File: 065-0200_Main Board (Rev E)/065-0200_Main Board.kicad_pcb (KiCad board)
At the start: 2 copper layers, 152.5 x 54.6 mm, 22 parts, among them J1 UJ32-C-H-G-H2-SMT-TR, J2 0022035025, J3 0022035025, J4 custom_3p_2mm, J5 custom_2p_2mm, SW1 3-1437565-0, U1 QRE1113GR, U2 QRE1113GR, U3 QRE1113GR, U4 BM833, U5 2SMPP03

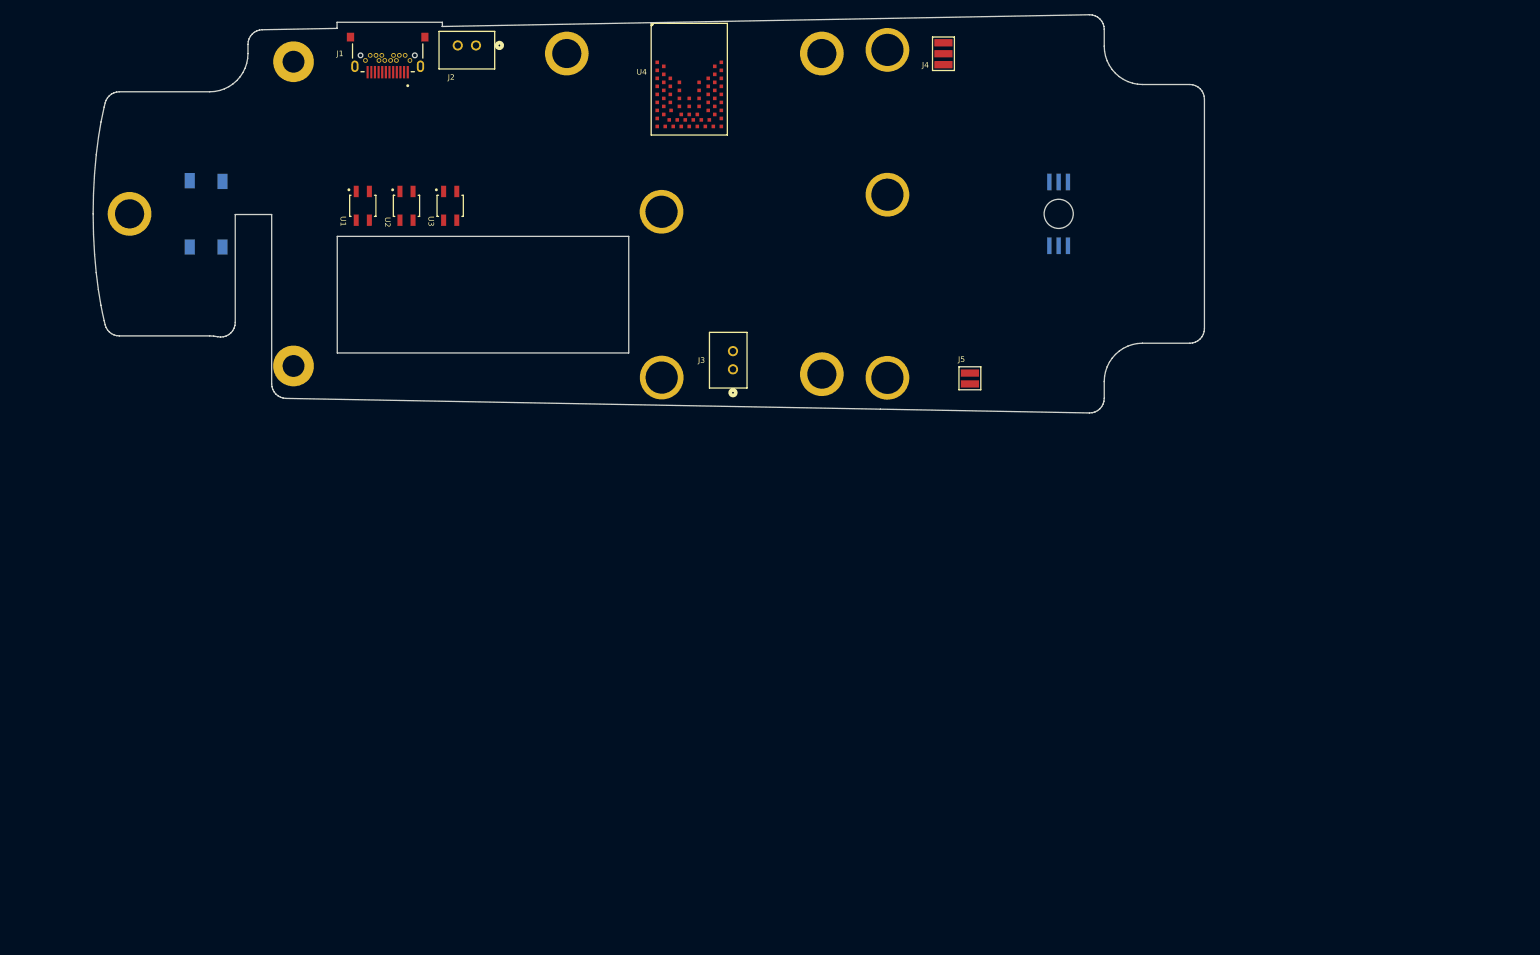
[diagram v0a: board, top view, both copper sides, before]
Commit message: Place all 155 remaining components on B.Cu off-board
Components grouped by circuit function below/around the board outline,
ready for manual placement. All on B.Cu with layers flipped F↔B.

Co-Authored-By: Claude Sonnet 4.6 <noreply@anthropic.com>
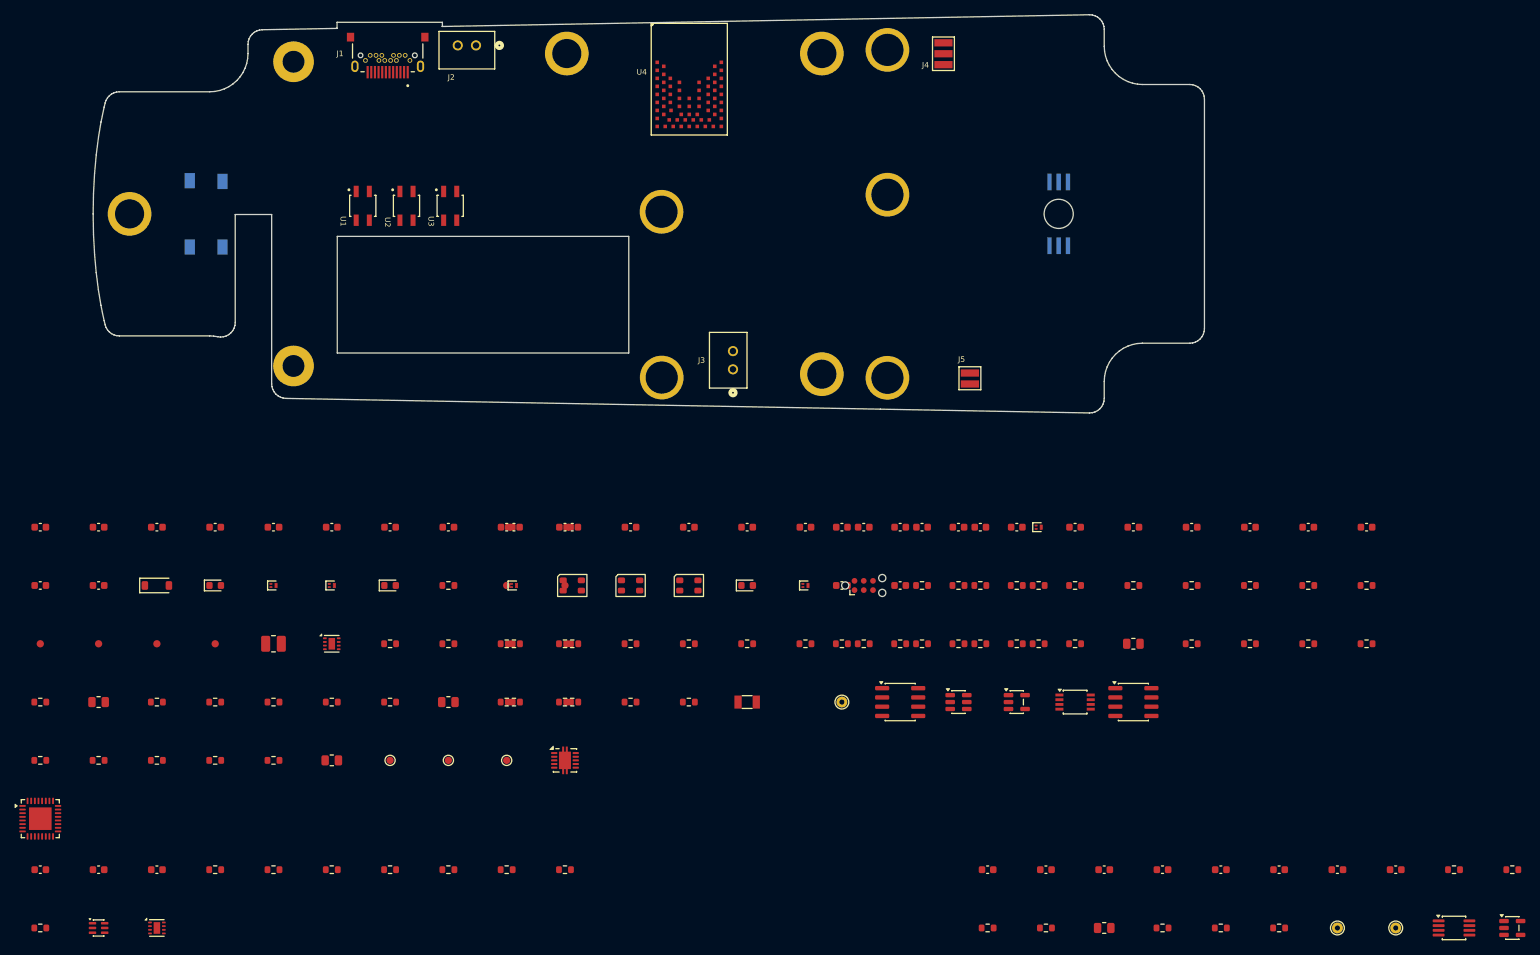
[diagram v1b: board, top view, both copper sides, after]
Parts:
- added C1: C_0603_1608Metric, Capacitor_SMD:C_0603_1608Metric, B.Cu at (65.0, 148.0)
- added C10: C_0603_1608Metric, Capacitor_SMD:C_0603_1608Metric, B.Cu at (73.0, 148.0)
- added C11: C_0603_1608Metric, Capacitor_SMD:C_0603_1608Metric, B.Cu at (195.0, 195.0)
- added C12: C_0603_1608Metric, Capacitor_SMD:C_0603_1608Metric, B.Cu at (203.0, 195.0)
- added C13: C_0603_1608Metric, Capacitor_SMD:C_0603_1608Metric, B.Cu at (211.0, 195.0)
- added C14: C_0603_1608Metric, Capacitor_SMD:C_0603_1608Metric, B.Cu at (175.0, 148.0)
- added C15: C_0603_1608Metric, Capacitor_SMD:C_0603_1608Metric, B.Cu at (183.0, 148.0)
- added C16: C_0603_1608Metric, Capacitor_SMD:C_0603_1608Metric, B.Cu at (219.0, 195.0)
- added C17: C_0603_1608Metric, Capacitor_SMD:C_0603_1608Metric, B.Cu at (191.0, 148.0)
- added C18: C_0603_1608Metric, Capacitor_SMD:C_0603_1608Metric, B.Cu at (199.0, 148.0)
- added C19: C_0603_1608Metric, Capacitor_SMD:C_0603_1608Metric, B.Cu at (207.0, 148.0)
- added C2: C_0603_1608Metric, Capacitor_SMD:C_0603_1608Metric, B.Cu at (81.0, 148.0)
- added C20: C_0603_1608Metric, Capacitor_SMD:C_0603_1608Metric, B.Cu at (215.0, 148.0)
- added C21: C_0603_1608Metric, Capacitor_SMD:C_0603_1608Metric, B.Cu at (227.0, 195.0)
- added C22: C_0603_1608Metric, Capacitor_SMD:C_0603_1608Metric, B.Cu at (223.0, 148.0)
- added C23: C_0603_1608Metric, Capacitor_SMD:C_0603_1608Metric, B.Cu at (231.0, 148.0)
- added C24: C_0603_1608Metric, Capacitor_SMD:C_0603_1608Metric, B.Cu at (235.0, 195.0)
- added C25: C_0603_1608Metric, Capacitor_SMD:C_0603_1608Metric, B.Cu at (243.0, 195.0)
- added C26: C_0603_1608Metric, Capacitor_SMD:C_0603_1608Metric, B.Cu at (239.0, 148.0)
- added C27: C_0603_1608Metric, Capacitor_SMD:C_0603_1608Metric, B.Cu at (247.0, 148.0)
- added C28: C_0603_1608Metric, Capacitor_SMD:C_0603_1608Metric, B.Cu at (251.0, 195.0)
- added C29: C_0603_1608Metric, Capacitor_SMD:C_0603_1608Metric, B.Cu at (175.0, 156.0)
- added C3: C_0603_1608Metric, Capacitor_SMD:C_0603_1608Metric, B.Cu at (130.0, 148.0)
- added C30: C_0603_1608Metric, Capacitor_SMD:C_0603_1608Metric, B.Cu at (89.0, 148.0)
- added C31: C_0603_1608Metric, Capacitor_SMD:C_0603_1608Metric, B.Cu at (97.0, 148.0)
- added C32: C_0603_1608Metric, Capacitor_SMD:C_0603_1608Metric, B.Cu at (183.0, 156.0)
- added C33: C_0603_1608Metric, Capacitor_SMD:C_0603_1608Metric, B.Cu at (105.0, 148.0)
- added C34: C_0603_1608Metric, Capacitor_SMD:C_0603_1608Metric, B.Cu at (113.0, 148.0)
- added C35: C_0603_1608Metric, Capacitor_SMD:C_0603_1608Metric, B.Cu at (121.0, 148.0)
- added C36: C_0603_1608Metric, Capacitor_SMD:C_0603_1608Metric, B.Cu at (129.0, 148.0)
- added C37: C_0603_1608Metric, Capacitor_SMD:C_0603_1608Metric, B.Cu at (137.0, 148.0)
- added C38: C_0603_1608Metric, Capacitor_SMD:C_0603_1608Metric, B.Cu at (138.0, 148.0)
- added C39: C_0603_1608Metric, Capacitor_SMD:C_0603_1608Metric, B.Cu at (146.0, 148.0)
- added C4: C_0603_1608Metric, Capacitor_SMD:C_0603_1608Metric, B.Cu at (154.0, 148.0)
- added C40: C_0603_1608Metric, Capacitor_SMD:C_0603_1608Metric, B.Cu at (162.0, 148.0)
- added C41: C_0603_1608Metric, Capacitor_SMD:C_0603_1608Metric, B.Cu at (65.0, 195.0)
- added C42: C_0603_1608Metric, Capacitor_SMD:C_0603_1608Metric, B.Cu at (73.0, 195.0)
- added C43: C_0603_1608Metric, Capacitor_SMD:C_0603_1608Metric, B.Cu at (81.0, 195.0)
- added C44: C_0603_1608Metric, Capacitor_SMD:C_0603_1608Metric, B.Cu at (65.0, 156.0)
- added C5: C_0603_1608Metric, Capacitor_SMD:C_0603_1608Metric, B.Cu at (170.0, 148.0)
- added C6: C_0603_1608Metric, Capacitor_SMD:C_0603_1608Metric, B.Cu at (178.0, 148.0)
- added C7: C_0603_1608Metric, Capacitor_SMD:C_0603_1608Metric, B.Cu at (186.0, 148.0)
- added C8: C_0603_1608Metric, Capacitor_SMD:C_0603_1608Metric, B.Cu at (194.0, 148.0)
- added C9: C_0603_1608Metric, Capacitor_SMD:C_0603_1608Metric, B.Cu at (73.0, 156.0)
- added D1: D_SOD-123, Diode_SMD:D_SOD-123, B.Cu at (81.0, 156.0)
- added D10: SOT-883, Package_TO_SOT_SMD:SOT-883, B.Cu at (202.0, 148.0)
- added D11: SOT-883, Package_TO_SOT_SMD:SOT-883, B.Cu at (130.0, 156.0)
- added D12: LED_0603_1608Metric, LED_SMD:LED_0603_1608Metric, B.Cu at (89.0, 156.0)
- added D2: SOT-883, Package_TO_SOT_SMD:SOT-883, B.Cu at (97.0, 156.0)
- added D3: SOT-883, Package_TO_SOT_SMD:SOT-883, B.Cu at (105.0, 156.0)
- added D4: LED_Cree-PLCC4_3.2x2.8mm_CCW, LED_SMD:LED_Cree-PLCC4_3.2x2.8mm_CCW, B.Cu at (138.0, 156.0)
- added D5: LED_Cree-PLCC4_3.2x2.8mm_CCW, LED_SMD:LED_Cree-PLCC4_3.2x2.8mm_CCW, B.Cu at (146.0, 156.0)
- added D6: LED_Cree-PLCC4_3.2x2.8mm_CCW, LED_SMD:LED_Cree-PLCC4_3.2x2.8mm_CCW, B.Cu at (154.0, 156.0)
- added D7: LED_0603_1608Metric, LED_SMD:LED_0603_1608Metric, B.Cu at (113.0, 156.0)
- added D8: LED_0603_1608Metric, LED_SMD:LED_0603_1608Metric, B.Cu at (162.0, 156.0)
- added D9: SOT-883, Package_TO_SOT_SMD:SOT-883, B.Cu at (170.0, 156.0)
- added F1: R_0603_1608Metric, Resistor_SMD:R_0603_1608Metric, B.Cu at (121.0, 156.0)
- added FD1: Fiducial_1mm_Mask2mm, Fiducial:Fiducial_1mm_Mask2mm, B.Cu at (129.0, 156.0)
- added FD2: Fiducial_1mm_Mask2mm, Fiducial:Fiducial_1mm_Mask2mm, B.Cu at (137.0, 156.0)
- added FD3: Fiducial_1mm_Mask2mm, Fiducial:Fiducial_1mm_Mask2mm, B.Cu at (65.0, 164.0)
- added FD4: Fiducial_1mm_Mask2mm, Fiducial:Fiducial_1mm_Mask2mm, B.Cu at (73.0, 164.0)
- added FD5: Fiducial_1mm_Mask2mm, Fiducial:Fiducial_1mm_Mask2mm, B.Cu at (81.0, 164.0)
- added FD6: Fiducial_1mm_Mask2mm, Fiducial:Fiducial_1mm_Mask2mm, B.Cu at (89.0, 164.0)
- added J6: Tag-Connect_TC2030-IDC-NL_2x03_P1.27mm_Vertical, Connector:Tag-Connect_TC2030-IDC-NL_2x03_P1.27mm_Vertical, B.Cu at (178.0, 156.0)
- added L1: L_1008_2520Metric, Inductor_SMD:L_1008_2520Metric, B.Cu at (97.0, 164.0)
- added Q1: WSON-8-1EP_2x2mm_P0.5mm_EP0.9x1.6mm, Package_SON:WSON-8-1EP_2x2mm_P0.5mm_EP0.9x1.6mm, B.Cu at (105.0, 164.0)
- added R1: R_0603_1608Metric, Resistor_SMD:R_0603_1608Metric, B.Cu at (113.0, 164.0)
- added R10: R_0603_1608Metric, Resistor_SMD:R_0603_1608Metric, B.Cu at (186.0, 156.0)
- added R11: R_0603_1608Metric, Resistor_SMD:R_0603_1608Metric, B.Cu at (194.0, 156.0)
- added R12: R_0603_1608Metric, Resistor_SMD:R_0603_1608Metric, B.Cu at (202.0, 156.0)
- added R13: R_0603_1608Metric, Resistor_SMD:R_0603_1608Metric, B.Cu at (130.0, 164.0)
- added R14: R_0603_1608Metric, Resistor_SMD:R_0603_1608Metric, B.Cu at (138.0, 164.0)
- added R15: R_0603_1608Metric, Resistor_SMD:R_0603_1608Metric, B.Cu at (146.0, 164.0)
- added R16: R_0603_1608Metric, Resistor_SMD:R_0603_1608Metric, B.Cu at (154.0, 164.0)
- added R17: R_0603_1608Metric, Resistor_SMD:R_0603_1608Metric, B.Cu at (162.0, 164.0)
- added R18: R_0603_1608Metric, Resistor_SMD:R_0603_1608Metric, B.Cu at (191.0, 156.0)
- added R19: R_0603_1608Metric, Resistor_SMD:R_0603_1608Metric, B.Cu at (199.0, 156.0)
- added R2: R_0603_1608Metric, Resistor_SMD:R_0603_1608Metric, B.Cu at (121.0, 164.0)
- added R20: R_0603_1608Metric, Resistor_SMD:R_0603_1608Metric, B.Cu at (259.0, 195.0)
- added R21: R_0603_1608Metric, Resistor_SMD:R_0603_1608Metric, B.Cu at (267.0, 195.0)
- added R22: R_0603_1608Metric, Resistor_SMD:R_0603_1608Metric, B.Cu at (207.0, 156.0)
- added R23: R_0603_1608Metric, Resistor_SMD:R_0603_1608Metric, B.Cu at (195.0, 203.0)
- added R24: R_0603_1608Metric, Resistor_SMD:R_0603_1608Metric, B.Cu at (203.0, 203.0)
- added R25: R_0603_1608Metric, Resistor_SMD:R_0603_1608Metric, B.Cu at (215.0, 156.0)
- added R26: R_0603_1608Metric, Resistor_SMD:R_0603_1608Metric, B.Cu at (223.0, 156.0)
- added R27: R_0603_1608Metric, Resistor_SMD:R_0603_1608Metric, B.Cu at (231.0, 156.0)
- added R28: R_0603_1608Metric, Resistor_SMD:R_0603_1608Metric, B.Cu at (239.0, 156.0)
- added R29: R_0603_1608Metric, Resistor_SMD:R_0603_1608Metric, B.Cu at (247.0, 156.0)
- added R3: R_0603_1608Metric, Resistor_SMD:R_0603_1608Metric, B.Cu at (129.0, 164.0)
- added R30: R_0603_1608Metric, Resistor_SMD:R_0603_1608Metric, B.Cu at (175.0, 164.0)
- added R31: R_0603_1608Metric, Resistor_SMD:R_0603_1608Metric, B.Cu at (183.0, 164.0)
- added R32: R_0603_1608Metric, Resistor_SMD:R_0603_1608Metric, B.Cu at (191.0, 164.0)
- added R33: R_0603_1608Metric, Resistor_SMD:R_0603_1608Metric, B.Cu at (199.0, 164.0)
- added R34: R_0805_2012Metric, Resistor_SMD:R_0805_2012Metric, B.Cu at (211.0, 203.0)
- added R35: R_0603_1608Metric, Resistor_SMD:R_0603_1608Metric, B.Cu at (207.0, 164.0)
- added R36: R_0805_2012Metric, Resistor_SMD:R_0805_2012Metric, B.Cu at (215.0, 164.0)
- added R37: R_0603_1608Metric, Resistor_SMD:R_0603_1608Metric, B.Cu at (219.0, 203.0)
- added R38: R_0603_1608Metric, Resistor_SMD:R_0603_1608Metric, B.Cu at (223.0, 164.0)
- added R39: R_0603_1608Metric, Resistor_SMD:R_0603_1608Metric, B.Cu at (231.0, 164.0)
- added R4: R_0603_1608Metric, Resistor_SMD:R_0603_1608Metric, B.Cu at (170.0, 164.0)
- added R40: R_0603_1608Metric, Resistor_SMD:R_0603_1608Metric, B.Cu at (137.0, 164.0)
- added R41: R_0603_1608Metric, Resistor_SMD:R_0603_1608Metric, B.Cu at (65.0, 172.0)
- added R42: R_0805_2012Metric, Resistor_SMD:R_0805_2012Metric, B.Cu at (73.0, 172.0)
- added R43: R_0603_1608Metric, Resistor_SMD:R_0603_1608Metric, B.Cu at (239.0, 164.0)
- added R44: R_0603_1608Metric, Resistor_SMD:R_0603_1608Metric, B.Cu at (247.0, 164.0)
- added R45: R_0603_1608Metric, Resistor_SMD:R_0603_1608Metric, B.Cu at (81.0, 172.0)
- added R46: R_0603_1608Metric, Resistor_SMD:R_0603_1608Metric, B.Cu at (89.0, 172.0)
- added R47: R_0603_1608Metric, Resistor_SMD:R_0603_1608Metric, B.Cu at (97.0, 172.0)
- added R48: R_0603_1608Metric, Resistor_SMD:R_0603_1608Metric, B.Cu at (105.0, 172.0)
- added R49: R_0603_1608Metric, Resistor_SMD:R_0603_1608Metric, B.Cu at (113.0, 172.0)
- added R5: R_0603_1608Metric, Resistor_SMD:R_0603_1608Metric, B.Cu at (178.0, 164.0)
- added R50: R_0805_2012Metric, Resistor_SMD:R_0805_2012Metric, B.Cu at (121.0, 172.0)
- added R51: R_0603_1608Metric, Resistor_SMD:R_0603_1608Metric, B.Cu at (129.0, 172.0)
- added R52: R_0603_1608Metric, Resistor_SMD:R_0603_1608Metric, B.Cu at (137.0, 172.0)
- added R53: R_0603_1608Metric, Resistor_SMD:R_0603_1608Metric, B.Cu at (186.0, 164.0)
- added R54: R_0603_1608Metric, Resistor_SMD:R_0603_1608Metric, B.Cu at (65.0, 180.0)
- added R55: R_0603_1608Metric, Resistor_SMD:R_0603_1608Metric, B.Cu at (73.0, 180.0)
- added R56: R_0603_1608Metric, Resistor_SMD:R_0603_1608Metric, B.Cu at (81.0, 180.0)
- added R57: R_0603_1608Metric, Resistor_SMD:R_0603_1608Metric, B.Cu at (194.0, 164.0)
- added R58: R_0603_1608Metric, Resistor_SMD:R_0603_1608Metric, B.Cu at (202.0, 164.0)
- added R59: R_0603_1608Metric, Resistor_SMD:R_0603_1608Metric, B.Cu at (130.0, 172.0)
- added R6: R_0603_1608Metric, Resistor_SMD:R_0603_1608Metric, B.Cu at (138.0, 172.0)
- added R60: R_0603_1608Metric, Resistor_SMD:R_0603_1608Metric, B.Cu at (89.0, 195.0)
- added R61: R_0603_1608Metric, Resistor_SMD:R_0603_1608Metric, B.Cu at (97.0, 195.0)
- added R62: R_0603_1608Metric, Resistor_SMD:R_0603_1608Metric, B.Cu at (105.0, 195.0)
- added R63: R_0603_1608Metric, Resistor_SMD:R_0603_1608Metric, B.Cu at (113.0, 195.0)
- added R64: R_0603_1608Metric, Resistor_SMD:R_0603_1608Metric, B.Cu at (146.0, 172.0)
- added R65: R_0603_1608Metric, Resistor_SMD:R_0603_1608Metric, B.Cu at (121.0, 195.0)
- added R66: R_0603_1608Metric, Resistor_SMD:R_0603_1608Metric, B.Cu at (129.0, 195.0)
- added R67: R_0603_1608Metric, Resistor_SMD:R_0603_1608Metric, B.Cu at (137.0, 195.0)
- added R68: R_0603_1608Metric, Resistor_SMD:R_0603_1608Metric, B.Cu at (65.0, 203.0)
- added R69: R_0603_1608Metric, Resistor_SMD:R_0603_1608Metric, B.Cu at (89.0, 180.0)
- added R7: R_0603_1608Metric, Resistor_SMD:R_0603_1608Metric, B.Cu at (97.0, 180.0)
- added R70: R_0603_1608Metric, Resistor_SMD:R_0603_1608Metric, B.Cu at (227.0, 203.0)
- added R71: R_0603_1608Metric, Resistor_SMD:R_0603_1608Metric, B.Cu at (235.0, 203.0)
- added R8: R_0805_2012Metric, Resistor_SMD:R_0805_2012Metric, B.Cu at (105.0, 180.0)
- added R9: R_0603_1608Metric, Resistor_SMD:R_0603_1608Metric, B.Cu at (154.0, 172.0)
- added TP1: TestPoint_Pad_D1.0mm, TestPoint:TestPoint_Pad_D1.0mm, B.Cu at (113.0, 180.0)
- added TP2: TestPoint_Pad_D1.0mm, TestPoint:TestPoint_Pad_D1.0mm, B.Cu at (121.0, 180.0)
- added TP3: TestPoint_THTPad_D1.5mm_Drill0.7mm, TestPoint:TestPoint_THTPad_D1.5mm_Drill0.7mm, B.Cu at (175.0, 172.0)
- added TP4: TestPoint_THTPad_D1.5mm_Drill0.7mm, TestPoint:TestPoint_THTPad_D1.5mm_Drill0.7mm, B.Cu at (243.0, 203.0)
- added TP5: TestPoint_THTPad_D1.5mm_Drill0.7mm, TestPoint:TestPoint_THTPad_D1.5mm_Drill0.7mm, B.Cu at (251.0, 203.0)
- added TP7: TestPoint_Pad_D1.0mm, TestPoint:TestPoint_Pad_D1.0mm, B.Cu at (129.0, 180.0)
- added U10: MSOP-8_3x3mm_P0.65mm, Package_SO:MSOP-8_3x3mm_P0.65mm, B.Cu at (259.0, 203.0)
- added U11: SOT-23-5, Package_TO_SOT_SMD:SOT-23-5, B.Cu at (267.0, 203.0)
- added U12: SOIC-8_3.9x4.9mm_P1.27mm, Package_SO:SOIC-8_3.9x4.9mm_P1.27mm, B.Cu at (183.0, 172.0)
- added U13: SOT-23-6, Package_TO_SOT_SMD:SOT-23-6, B.Cu at (191.0, 172.0)
- added U14: VSON-10-1EP_3x3mm_P0.5mm_EP1.65x2.4mm, Package_SON:VSON-10-1EP_3x3mm_P0.5mm_EP1.65x2.4mm, B.Cu at (137.0, 180.0)
- added U15: QFN-32-1EP_5x5mm_P0.5mm_EP3.1x3.1mm, Package_DFN_QFN:QFN-32-1EP_5x5mm_P0.5mm_EP3.1x3.1mm, B.Cu at (65.0, 188.0)
- added U16: SOT-363_SC-70-6, Package_TO_SOT_SMD:SOT-363_SC-70-6, B.Cu at (73.0, 203.0)
- added U6: SOT-23-5, Package_TO_SOT_SMD:SOT-23-5, B.Cu at (199.0, 172.0)
- added U7: TSSOP-8_3x3mm_P0.65mm, Package_SO:TSSOP-8_3x3mm_P0.65mm, B.Cu at (207.0, 172.0)
- added U8: WSON-8-1EP_2x2mm_P0.5mm_EP0.9x1.6mm, Package_SON:WSON-8-1EP_2x2mm_P0.5mm_EP0.9x1.6mm, B.Cu at (81.0, 203.0)
- added U9: SOIC-8_3.9x4.9mm_P1.27mm, Package_SO:SOIC-8_3.9x4.9mm_P1.27mm, B.Cu at (215.0, 172.0)
- added Y1: Crystal_SMD_3215-2Pin_3.2x1.5mm, Crystal:Crystal_SMD_3215-2Pin_3.2x1.5mm, B.Cu at (162.0, 172.0)
